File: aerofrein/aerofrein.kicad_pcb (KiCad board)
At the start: 2 copper layers, 50 x 31 mm, 16 parts, among them J1 endstop, J2 HMI, J3 comm, J4 MSX, J5 power, J6 motor, U1 RP2040, U2 TMC2209

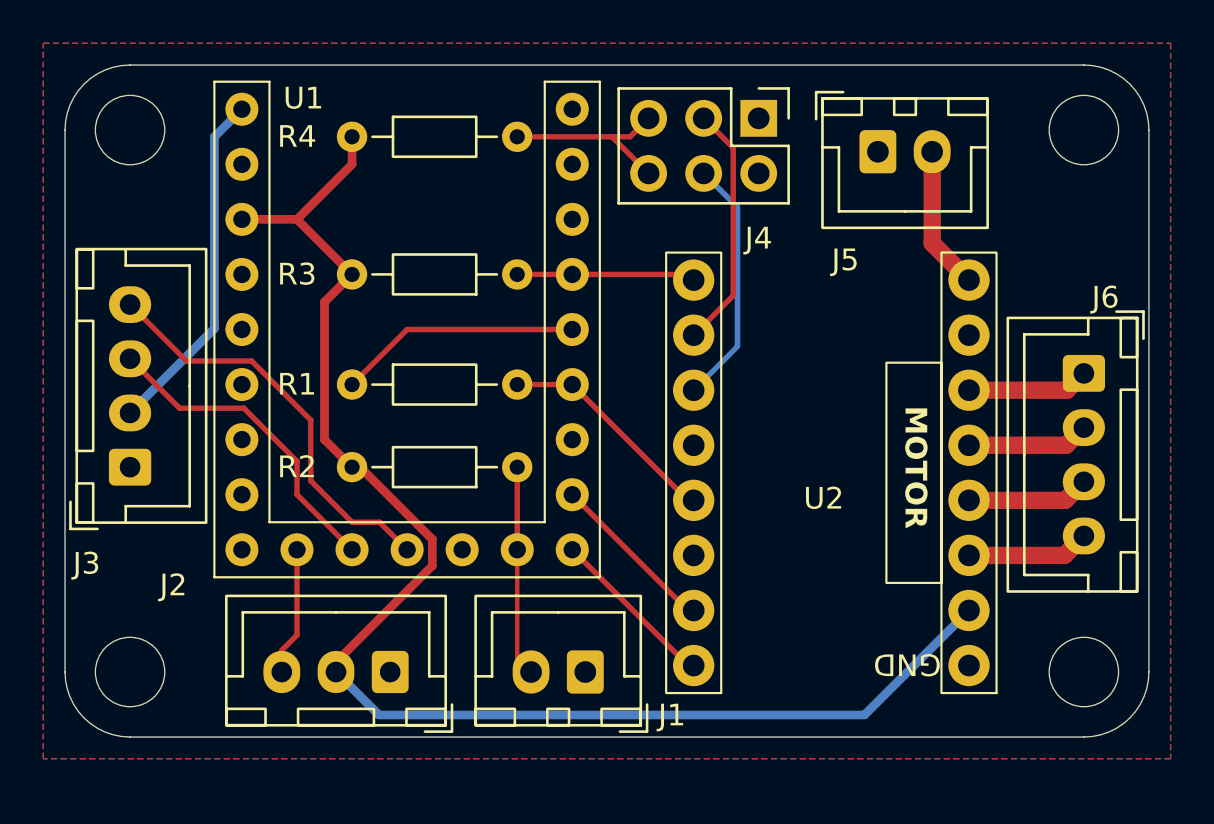
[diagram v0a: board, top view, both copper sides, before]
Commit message: airbrake full revision
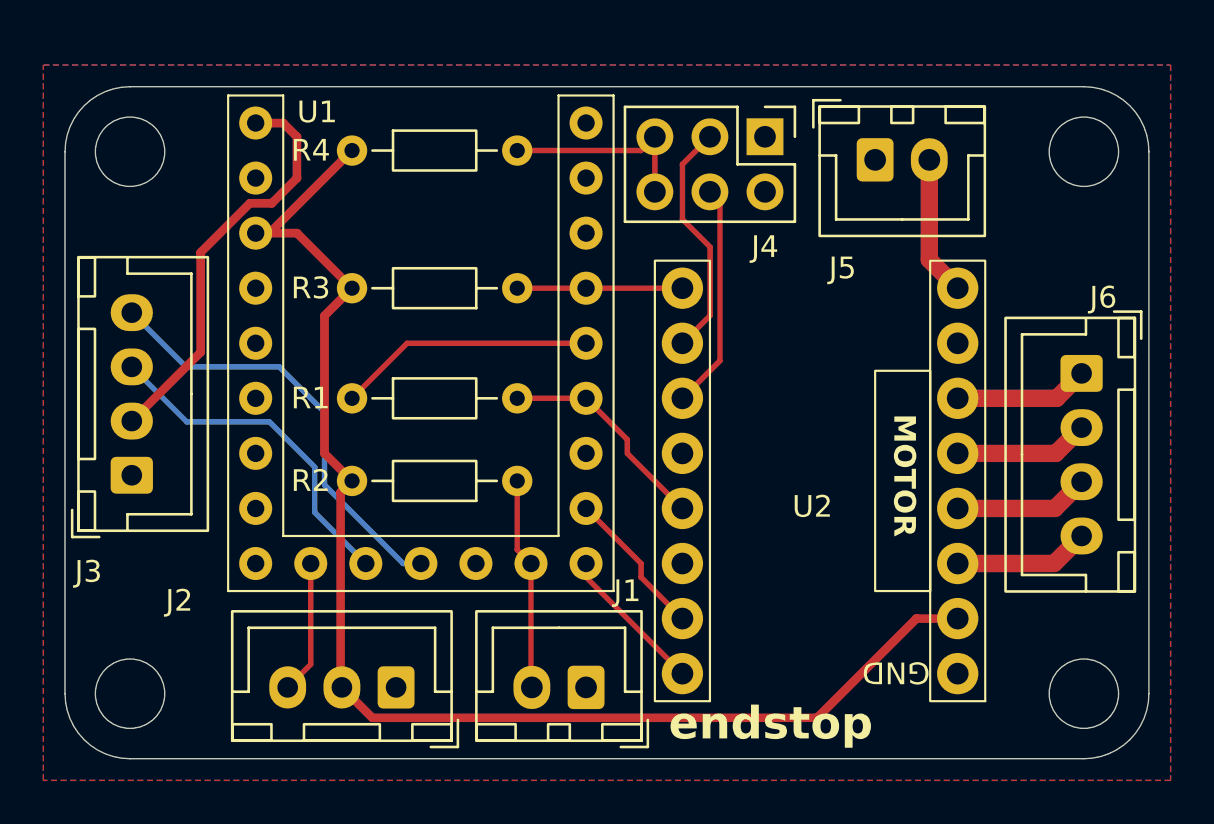
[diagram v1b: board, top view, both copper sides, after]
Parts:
- removed H2, H3, H4: MountingHole_3.2mm_M3_ISO7380, MountingHole:MountingHole_3.2mm_M3_ISO7380
- added H1: MountingHole_3.2mm_M3_ISO7380, MountingHole:MountingHole_3.2mm_M3_ISO7380, F.Cu at (132.0, 93.0)
- added H1: MountingHole_3.2mm_M3_ISO7380, MountingHole:MountingHole_3.2mm_M3_ISO7380, F.Cu at (176.0, 93.0)
- added H1: MountingHole_3.2mm_M3_ISO7380, MountingHole:MountingHole_3.2mm_M3_ISO7380, F.Cu at (176.0, 68.0)
- moved H1 1.00 mm to (132.0, 68.0)
- moved J4 0.90 mm to (161.3, 67.3)
- moved U1 0.90 mm to (145.4, 66.7)
- moved J2 0.76 mm to (144.3, 92.7)
- moved J1 0.71 mm to (153.0, 92.7)
- moved U2 0.64 mm to (162.6, 97.2)
- moved R1 0.64 mm to (142.2, 79.4)
- moved R2 0.64 mm to (149.9, 83.2)
- moved R3 0.64 mm to (149.9, 74.3)
- moved R4 0.63 mm to (142.2, 67.9)
- moved J5 0.40 mm to (166.4, 68.4)
- moved J3 0.38 mm to (132.1, 82.9)
- moved J6 0.10 mm to (175.9, 78.2)
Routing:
- net +3V3: track 66.0 -> 61.5 mm
- net +5V: track 16.1 -> 19.0 mm
- net /MS2: track 11.5 -> 10.4 mm
- net /SCL: track 14.8 -> 15.8 mm
- net /SDA: track 19.1 -> 20.1 mm
- net /TMC_STEP: track 7.81 -> 6.92 mm
- net /TMC_DIR: track 7.81 -> 6.92 mm
- net Net-(U1-GPIO4): track 11.2 -> 11.8 mm
- net /TMC_EN: track 8.25 -> 7.62 mm
- net Net-(J6-Pin_4): track 5.67 -> 6.24 mm
- net Net-(J6-Pin_2): track 5.64 -> 6.21 mm
- net Net-(J6-Pin_1): track 5.62 -> 6.19 mm
- net Net-(J6-Pin_3): track 5.65 -> 6.22 mm
